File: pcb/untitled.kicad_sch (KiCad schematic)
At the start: 2 parts

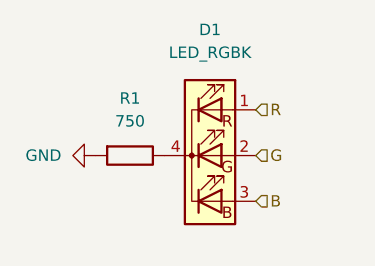
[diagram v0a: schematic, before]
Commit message: asigning the footprints
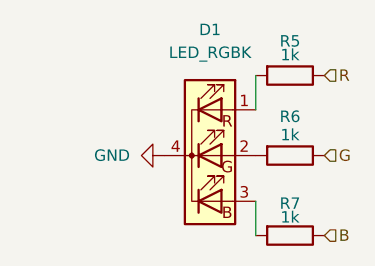
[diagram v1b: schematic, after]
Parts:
- removed R1: 750, Package_SON:Winbond_USON-8-1EP_3x2mm_P0.5mm_EP0.2x1.6mm, symbol Device:R
- added R5, R6, R7: 1k, Resistor_SMD:R_0603_1608Metric, symbol Device:R
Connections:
- net B: now also R7.1; no longer D1.3 (BA)
- net G: now also R6.1; no longer D1.2 (GA)
- net GND: now also D1.4 (K)
- net R: now also R5.1; no longer D1.1 (RA)
- new net: D1.1 (RA), R5.2
- new net: D1.3 (BA), R7.2
- new net: D1.2 (GA), R6.2

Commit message: asigning the part numbers
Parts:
- D1: footprint LED_SMD:LED_ASMB-KTF0-0A306 -> LED_SMD:LED_WS2812B_PLCC4_5.0x5.0mm_P3.2mm; LCSC Part (none) -> C52917433
- R5, R6, R7: LCSC Part (none) -> C22548
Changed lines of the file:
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@@
+			)
+		)
+		(property "LCSC Part" "C22548"
+			(at 168.91 83.82 90)
+			(hide yes)
+			(show_name no)
+			(do_not_autoplace no)
+			(effects
+				(font
+					(size 1.27 1.27)
+				)
 			)
 		)
@@
 			)
 		)
+		(property "LCSC Part" "C22548"
+			(at 168.91 101.6 90)
+			(hide yes)
+			(show_name no)
+			(do_not_autoplace no)
+			(effects
+				(font
+					(size 1.27 1.27)
+				)
+			)
+		)
 		(pin "1"
 		)
@@
 		)
 		(property "KLC_S4.2_VREG_VOUT" ""
+			(at 168.91 92.71 90)
+			(hide yes)
+			(show_name no)
+			(do_not_autoplace no)
+			(effects
+				(font
+					(size 1.27 1.27)
+				)
+			)
+		)
+		(property "LCSC Part" "C22548"
 			(at 168.91 92.71 90)
 			(hide yes)
@@
 			)
 		)
-		(property "Footprint" "LED_SMD:LED_ASMB-KTF0-0A306"
+		(property "Footprint" "LED_SMD:LED_WS2812B_PLCC4_5.0x5.0mm_P3.2mm"
 			(at 160.02 93.98 0)
 			(hide yes)
@@
 			(at 160.02 92.71 0)
 			(hide yes)
+			(show_name no)
+			(do_not_autoplace no)
+			(effects
+				(font
+					(size 1.27 1.27)
+				)
+			)
+		)
+		(property "LCSC Part" "C52917433"
+			(at 160.02 92.71 0)
+			(hide yes)
